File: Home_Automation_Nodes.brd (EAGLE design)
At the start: 122.7 x 69.5 mm, 19 parts

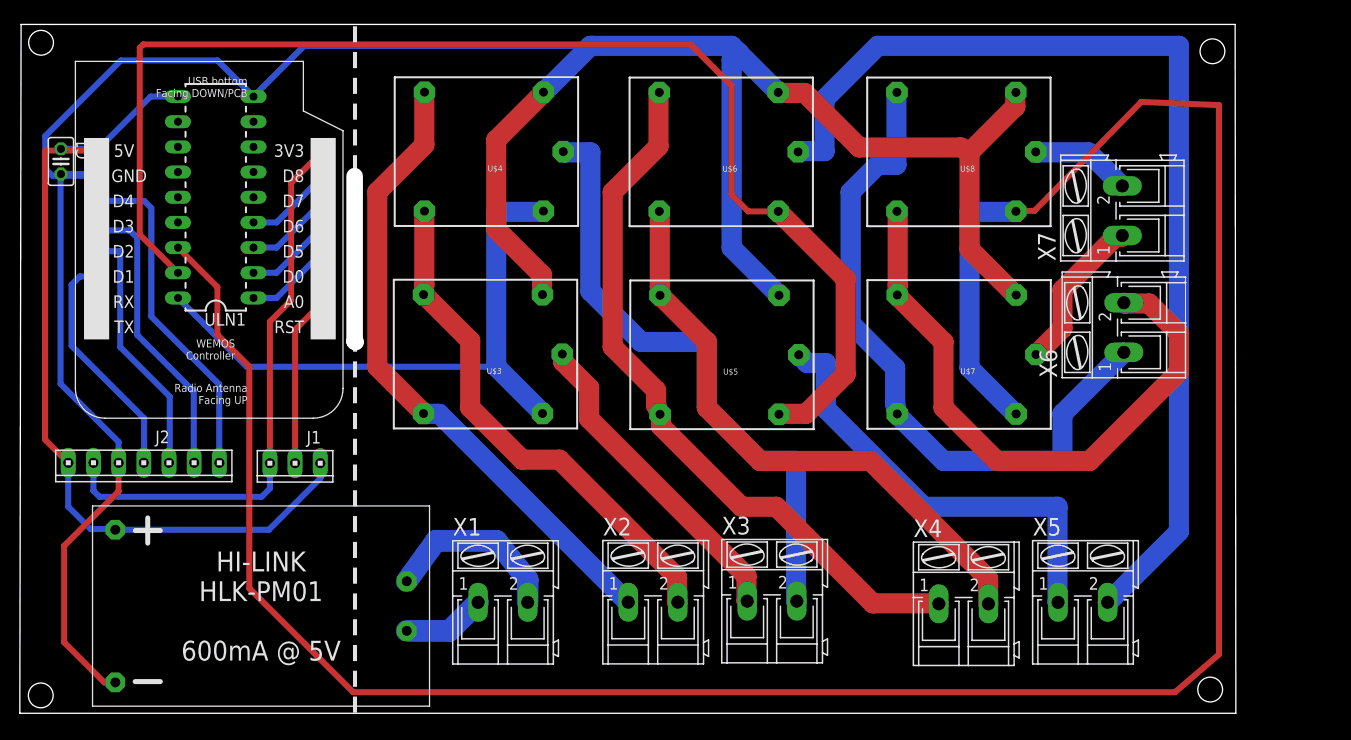
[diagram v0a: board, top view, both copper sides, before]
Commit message: Final version. Sent to Mervin for verification
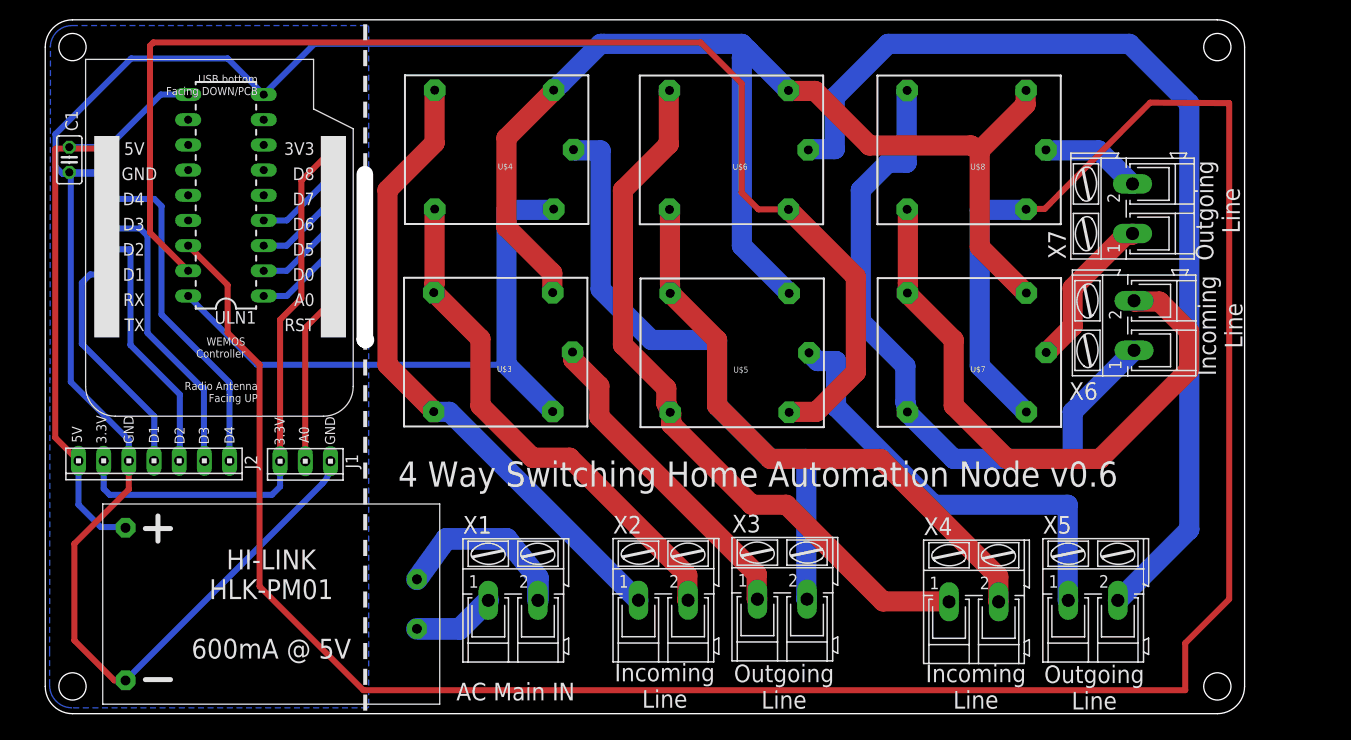
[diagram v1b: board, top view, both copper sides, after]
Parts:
- moved U$3 1.05 mm to (45.8, 36.4)
- moved U$4 1.05 mm to (45.9, 56.8)
- moved U$7 1.05 mm to (93.6, 36.3)
- moved U$8 1.05 mm to (93.6, 56.8)
- moved ULN1 1.05 mm to (18.2, 52.3)
- moved X7 1.05 mm to (109.7, 51.0)
- moved U$2 1.05 mm to (22.8, 11.1)
- moved X1 1.05 mm to (47.2, 11.4)
- moved X2 1.05 mm to (62.4, 11.4)
- moved X3 1.05 mm to (74.4, 11.6)
- moved X4 1.05 mm to (93.7, 11.3)
- moved X5 1.05 mm to (105.7, 11.4)
- moved U$5 1.05 mm to (69.7, 36.3)
- moved U$6 1.05 mm to (69.6, 56.8)
- moved X6 1.05 mm to (109.8, 39.2)
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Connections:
- net 5V: no longer J1.3
- net GND: now also J1.3
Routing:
- net GND: track 258.0 -> 288.8 mm
- net 5V: track 86.3 -> 62.1 mm
- net N$18: track 105.1 -> 101.7 mm
- added copper zone on layer 16, net GND
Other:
- board size 122.7 x 69.5 mm -> 121 x 70 mm
- board text added: "3.3V"
- board text added: "4 Way Switching Home Automation Node v0.6"
- board text added: "5V"
- board text added: "A0"
- board text added: "D1"
- board text added: "D2"
- board text added: "D3"
- board text added: "D4"
- board text added: "GND"
- board text added: "Outgoing Line"
- board text removed: "Outcoming Line"
